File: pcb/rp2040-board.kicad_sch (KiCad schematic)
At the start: 6 parts, among them U1 RP2040, U2 W25Q128JVS

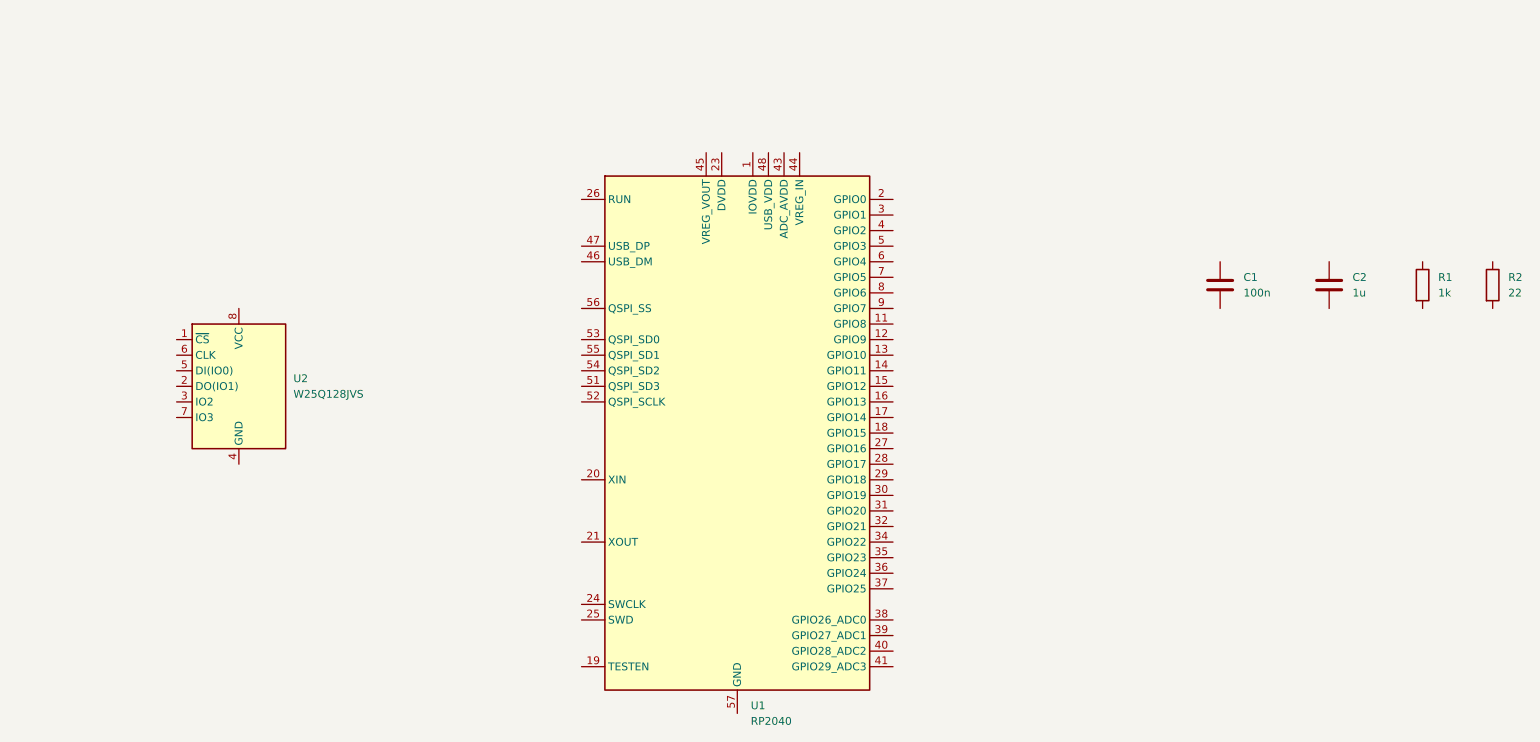
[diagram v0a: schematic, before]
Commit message: schematic wip
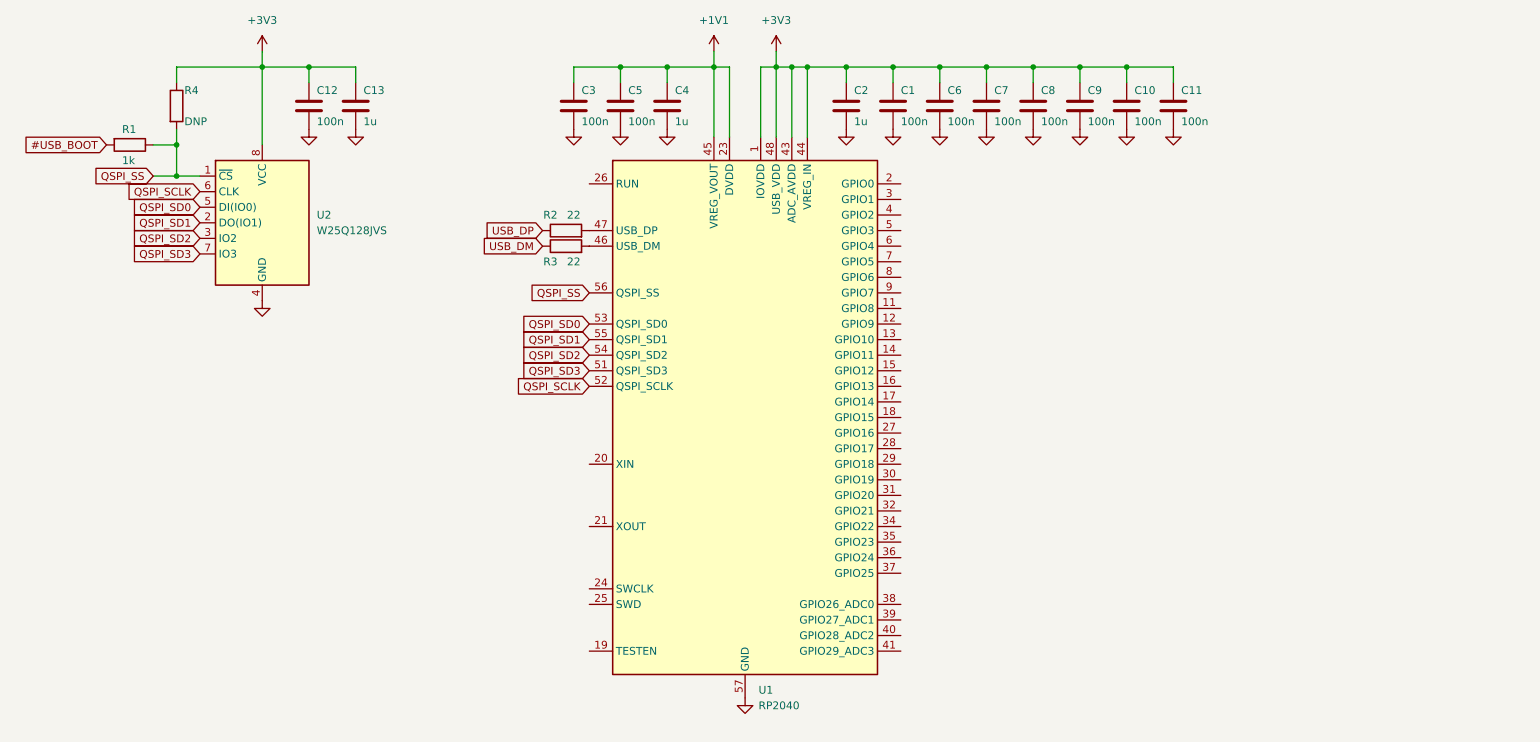
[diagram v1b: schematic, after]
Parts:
- added C10, C11, C12, C3, C5, C6, C7, C8, C9: 100n, Capacitor_SMD:C_0402_1005Metric, symbol Device:C
- added C13, C4: 1u, Capacitor_SMD:C_0402_1005Metric, symbol Device:C
- added R3: 22, Resistor_SMD:R_0402_1005Metric, symbol Device:R
- added R4: DNP, Resistor_SMD:R_0402_1005Metric, symbol Device:R
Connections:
- net QSPI_SS: now reaches U2.1 (~{CS})
- net QSPI_SS: now also R1.1, U1.56 (QSPI_SS), R4.2
- net QSPI_SD1: now reaches U2.2 (DO(IO1))
- net QSPI_SD1: now also U1.55 (QSPI_SD1)
- net QSPI_SD2: now reaches U2.3 (IO2)
- net QSPI_SD2: now also U1.54 (QSPI_SD2)
- net GND: now reaches U2.4 (GND)
- net GND: now also C1.2, C2.2, U1.57 (GND), C10.2, C11.2, C12.2, C13.2, C3.2, C4.2, C5.2, C6.2, C7.2, C8.2, C9.2
- net QSPI_SD0: now reaches U2.5 (DI(IO0))
- net QSPI_SD0: now also U1.53 (QSPI_SD0)
- net QSPI_SCLK: now reaches U2.6 (CLK)
- net QSPI_SCLK: now also U1.52 (QSPI_SCLK)
- net QSPI_SD3: now reaches U2.7 (IO3)
- net QSPI_SD3: now also U1.51 (QSPI_SD3)
- net +3V3: now reaches U2.8 (VCC)
- net +3V3: now also C1.1, C2.1, U1.1 (IOVDD), U1.10 (IOVDD), U1.22 (IOVDD), U1.33 (IOVDD), U1.42 (IOVDD), U1.43 (ADC_AVDD), U1.44 (VREG_IN), U1.48 (USB_VDD), U1.49 (IOVDD), C10.1, C11.1, C12.1, C13.1, C6.1, C7.1, C8.1, C9.1, R4.1
- net USB_DP: now reaches R2.1
- net at R2.2: now also U1.47 (USB_DP)
- net #USB_BOOT: now reaches R1.2
- net +1V1: now reaches U1.23 (DVDD), U1.50 (DVDD)
- net +1V1: now also U1.45 (VREG_VOUT), C3.1, C4.1, C5.1
- net at U1.46 (USB_DM): now also R3.2
- new net USB_DM: R3.1
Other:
- moved on the sheet: C1, C2, R1, R2, U1, U2
